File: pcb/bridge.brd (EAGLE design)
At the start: 99.4 x 59 mm, 46 parts, among them IC1 MEGA8-AI, IC4 78L05SMD, IC5 LM358D, Q1 16MHz, X1 PN61729-S

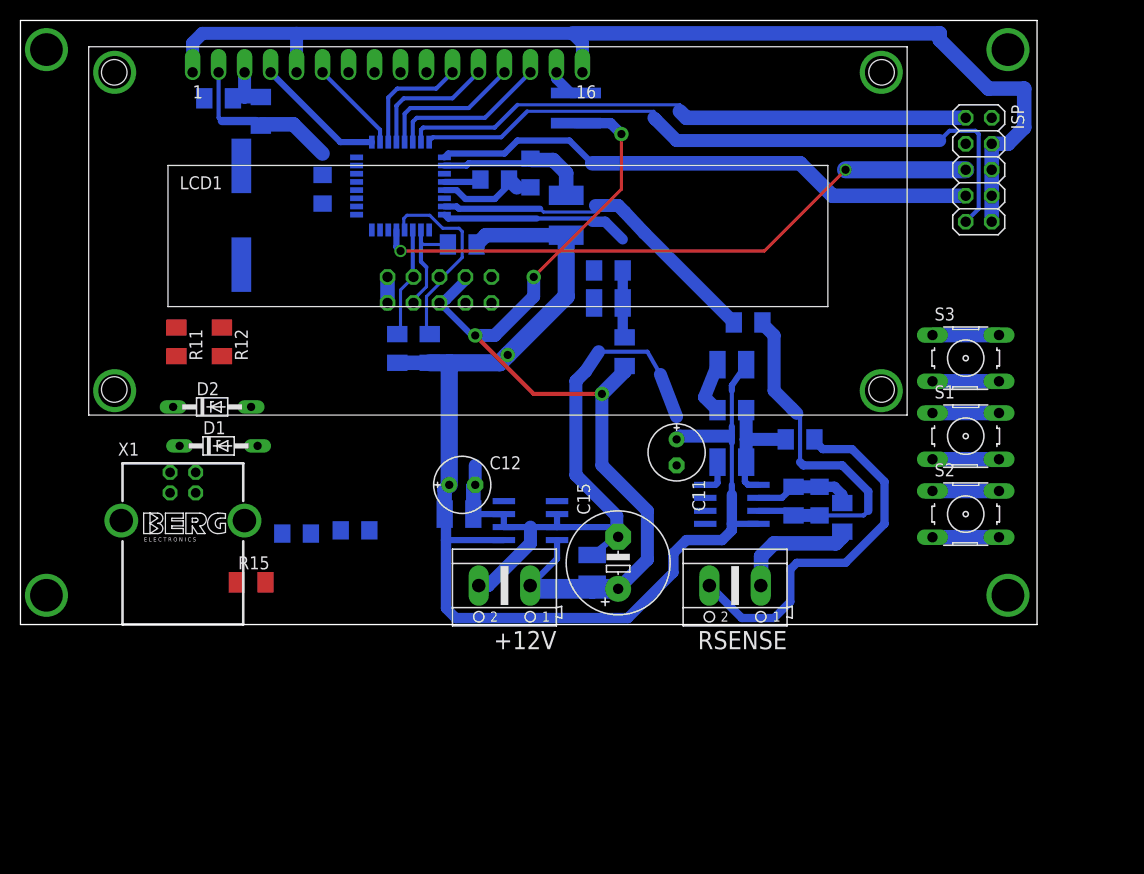
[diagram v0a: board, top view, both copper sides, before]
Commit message: Bridge board ready.
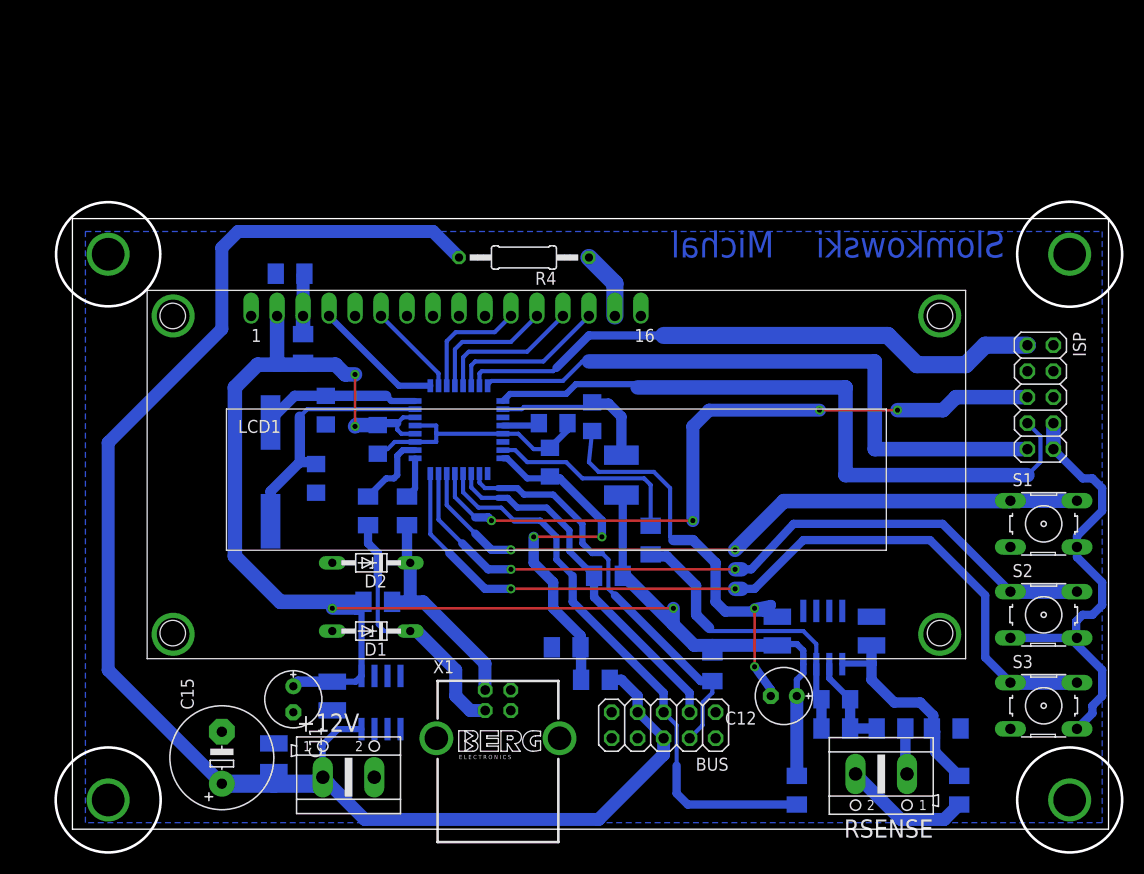
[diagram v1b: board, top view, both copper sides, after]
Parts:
- removed C17: 100n, rcl:C1210
- added C7: 100n, rcl:C1206
- R4: device rcl:R1218 -> rcl:0207/12
- moved R1 56.1 mm to (70.5, 4.76), turned to 90 degrees
- moved R3 48.0 mm to (62.2, 16.8), turned to 90 degrees
- moved BUS 47.9 mm to (57.5, 11.1), flipped to the top
- moved C11 44.6 mm to (21.3, 13.7)
- moved C15 43.2 mm to (14.3, 7.94)
- moved R6 37.7 mm to (86.4, 4.76), turned to 90 degrees
- moved C12 37.6 mm to (69.2, 14.0), turned to 180 degrees
- moved R8 37.5 mm to (85.1, 10.8), turned to 0 degrees
- moved X1 37.4 mm to (41.3, 9.84)
- moved R14 37.1 mm to (47.9, 18.7)
- moved C14 36.2 mm to (19.4, 7.94)
- moved S3 34.8 mm to (94.6, 13.0)
- moved R13 32.2 mm to (50.8, 15.6), turned to 180 degrees
- moved R2 30.3 mm to (52.1, 25.7), turned to 180 degrees
- moved R11 27.9 mm to (32.4, 32.1), flipped to the bottom
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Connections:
- removed net FDFDS: S1.1, S1.2
- removed net XXFDSF: S2.1, S2.2
- removed net XXX: S3.1, S3.2
- net GND: now also C7.2; no longer C17.2
- net PC1: now also C7.1; no longer C17.1
- net PD0: now also S1.1, S1.2
- net PD1: now also S2.1, S2.2
- net PD2: now also S3.1, S3.2
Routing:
- net GND: track 215.3 -> 113.4 mm, vias 0 -> 2
- net PD2: track 0.00 -> 82.6 mm, vias 0 -> 2
- net PD1: track 0.00 -> 74.2 mm, vias 0 -> 2
- net PD0: track 0.00 -> 68.5 mm, vias 0 -> 2
- net +12V: track 95.4 -> 153.2 mm, vias 4 -> 0
- net PC5: track 19.4 -> 54.9 mm
- net PC3: track 11.8 -> 41.0 mm
- net N$6: track 0.00 -> 25.6 mm
- net N$9: track 0.00 -> 24.6 mm
- net N$29: track 37.1 -> 12.6 mm
- net PC4: track 10.9 -> 35.3 mm
- net N$5: track 0.00 -> 21.8 mm
- net +5V: track 138.3 -> 157.3 mm, vias 1 -> 4
- net N$11: track 0.00 -> 15.6 mm
- net PC0: track 34.3 -> 19.8 mm
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- added copper zone on layer 16, net GND
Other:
- board size 99.4 x 59 mm -> 104.2 x 63.6 mm
- board text added: "Michal"
- board text added: "Slomkowski"
